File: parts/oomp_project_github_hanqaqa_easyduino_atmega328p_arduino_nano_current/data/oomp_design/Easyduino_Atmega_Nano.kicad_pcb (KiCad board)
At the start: 4 copper layers, 43.4 x 18 mm, 31 parts, among them J1 USB_C_Receptacle_USB2.0, J2 ICSP, SW1 SW_Push, U1 ATmega328P-A, U2 XC6206P502MR, U3 CP2102N-Axx-xQFN28, Y1 16 MHz

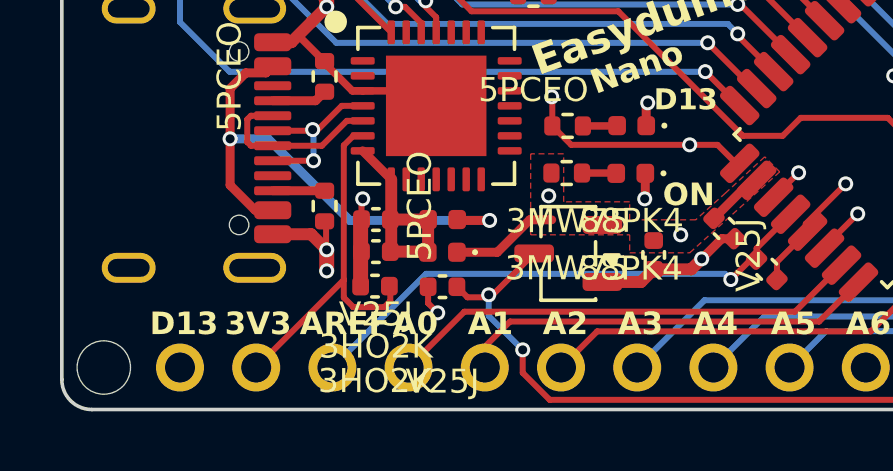
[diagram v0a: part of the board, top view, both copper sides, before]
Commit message: current
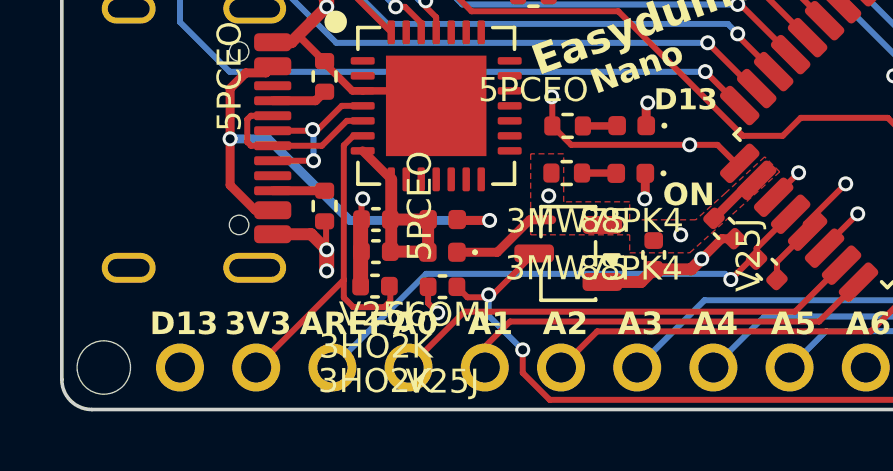
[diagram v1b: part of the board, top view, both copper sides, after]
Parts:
- F1: footprint Fuse:Fuse_0402_1005Metric -> OOMP_MachineSolder:electronic_fuse_0402_resettable

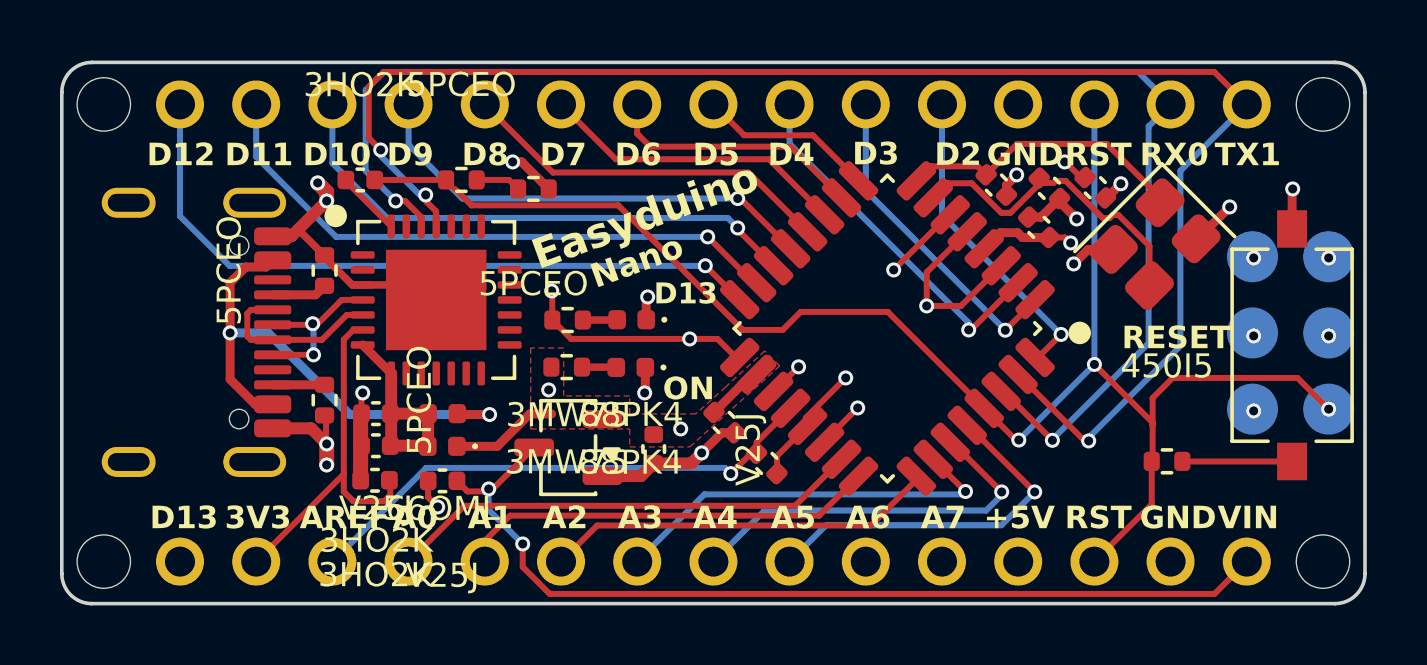
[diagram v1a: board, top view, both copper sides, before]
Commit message: working
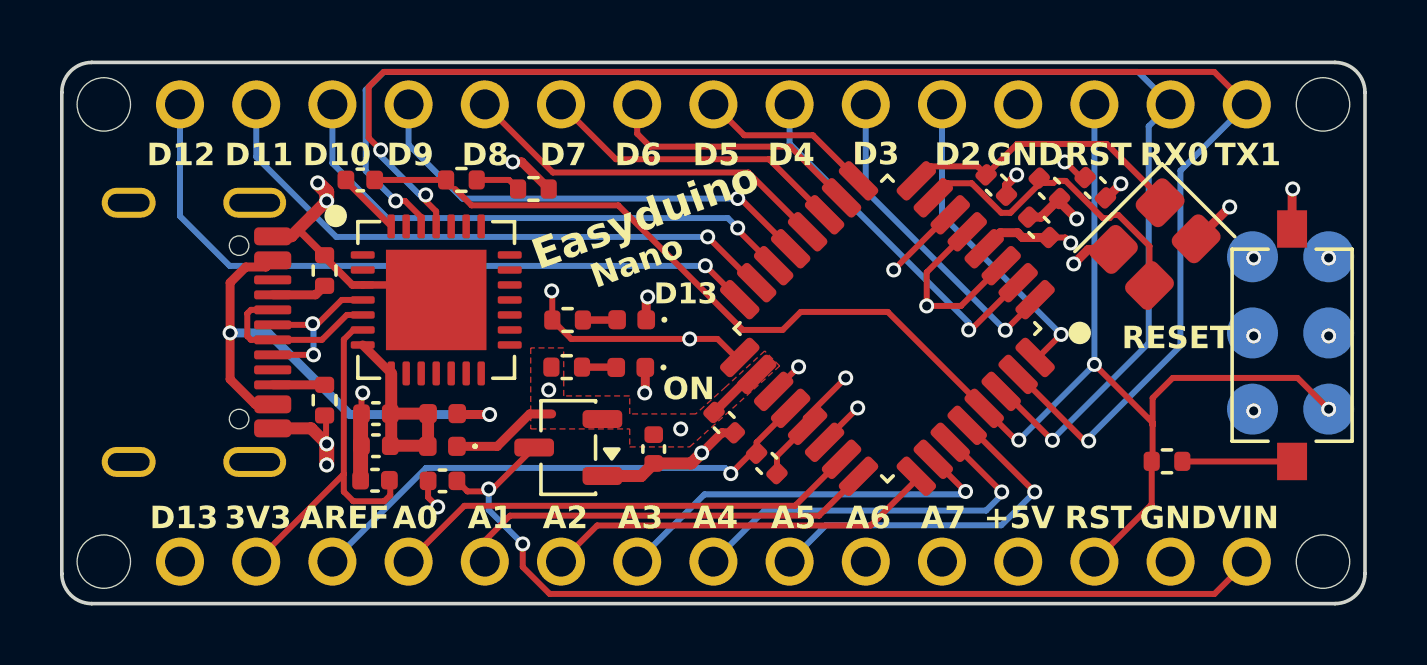
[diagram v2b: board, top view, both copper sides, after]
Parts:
- C1, C11, C12: footprint OOMP_MachineSolder:electronic_capacitor_0402_1_micro_farad -> Capacitor_SMD:C_0402_1005Metric
- C2, C3, C4: footprint OOMP_MachineSolder:electronic_capacitor_0402_100_nano_farad -> Capacitor_SMD:C_0402_1005Metric
- D1, D3: footprint OOMP_MachineSolder:electronic_led_0402 -> LED_SMD:LED_0402_1005Metric
- F1: footprint OOMP_MachineSolder:electronic_fuse_0402_resettable -> Fuse:Fuse_0402_1005Metric
- R1, R2, R3, R4: footprint OOMP_MachineSolder:electronic_resistor_0402_5100_ohm -> Resistor_SMD:R_0402_1005Metric
- R5: footprint OOMP_MachineSolder:electronic_resistor_0402_330_ohm -> Resistor_SMD:R_0402_1005Metric
- R6, R7: footprint OOMP_MachineSolder:electronic_resistor_0402_2000_ohm -> Resistor_SMD:R_0402_1005Metric
